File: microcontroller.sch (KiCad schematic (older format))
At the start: 52 parts, among them J3 FH12A-10S-0.5SH55, J4 , J5 Conn_ARM_JTAG_SWD_20, J6 26642801RP2, SW0 SW_Push, SW1 SW_Push, SW2 SW_Push, SW3 SW_Push, SW4 SW_Push, SW5 SW_Push, SW6 SW_Push, U7 EFM32GG942F1024

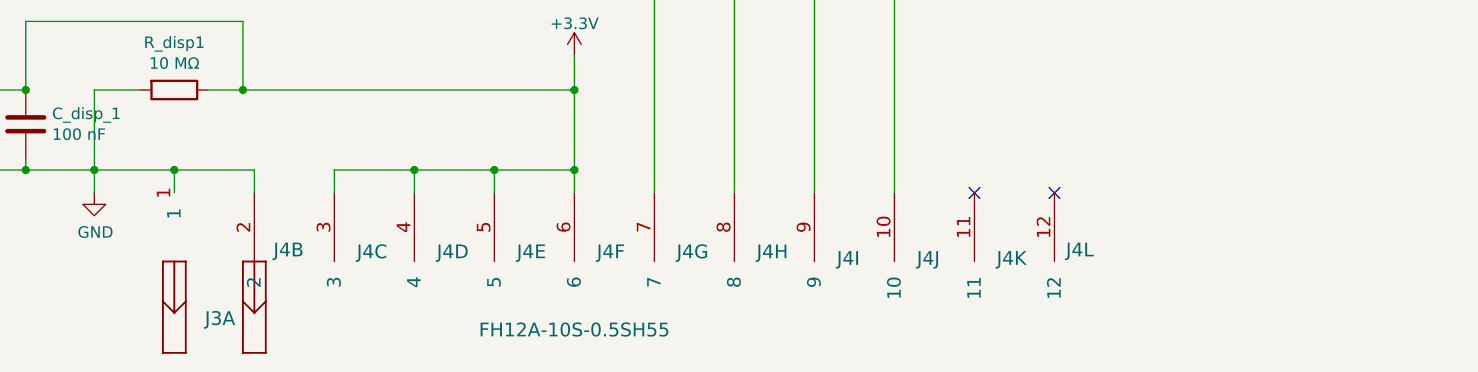
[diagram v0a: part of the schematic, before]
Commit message: Organize components and fix minor issues
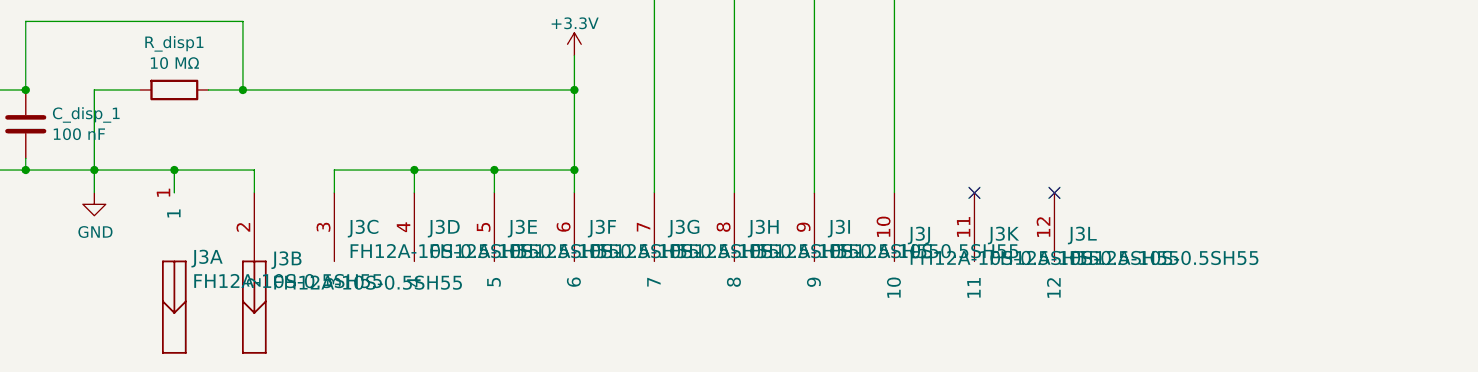
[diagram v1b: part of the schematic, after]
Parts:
- removed J4: (no value), Local:FH12A-10S-0.5SH55, symbol LCD:FH12A-10S-0.5SH55
- added unit 2 of J3
- added unit 3 of J3
- added unit 4 of J3
- added unit 5 of J3
- added unit 6 of J3
- added unit 7 of J3
- added unit 8 of J3
- added unit 9 of J3
- added unit 10 of J3
- added unit 11 of J3
- added unit 12 of J3
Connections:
- net +3V3: now also J3.3, J3.4, J3.5, J3.6
- net GND: now also J3.2
- net at U7.28 (PD0): now also J3.9
- net at U7.30 (PD2): now also J3.10
- net at U7.31 (PD3): now also J3.8
- net at J6.14: now also J3.7
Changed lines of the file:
@@
 	4400 6350 3800 6350
-$Comp
-L LCD:FH12A-10S-0.5SH55 J4
-U 2 1 5D873ACF
-P 4000 9050
-F 0 "J4" V 3750 9200 60  0000 C CNN
-F 1 " " V 4200 9050 60  0000 C CNN
-F 2 "Local:FH12A-10S-0.5SH55" H 4000 8990 60  0001 C CNN
-F 3 "" H 4000 9050 60  0000 C CNN
-	2    4000 9050
-	0    1    -1   0
-$EndComp
-$Comp
-L LCD:FH12A-10S-0.5SH55 J4
-U 3 1 5D88452F
-P 4350 9050
-F 0 "J4" V 4092 9148 60  0000 L CNN
-F 1 " " V 4198 9148 60  0000 L CNN
-F 2 "Local:FH12A-10S-0.5SH55" H 4350 8990 60  0001 C CNN
-F 3 "" H 4350 9050 60  0000 C CNN
-	3    4350 9050
-	0    1    -1   0
-$EndComp
-$Comp
-L LCD:FH12A-10S-0.5SH55 J4
-U 4 1 5D88BAB2
-P 4700 9050
-F 0 "J4" V 4442 9148 60  0000 L CNN
-F 1 " " V 4548 9148 60  0000 L CNN
-F 2 "Local:FH12A-10S-0.5SH55" H 4700 8990 60  0001 C CNN
-F 3 "" H 4700 9050 60  0000 C CNN
-	4    4700 9050
-	0    1    -1   0
-$EndComp
-$Comp
-L LCD:FH12A-10S-0.5SH55 J4
-U 5 1 5D891720
-P 5050 9050
-F 0 "J4" V 4792 9148 60  0000 L CNN
-F 1 " " V 4898 9148 60  0000 L CNN
-F 2 "Local:FH12A-10S-0.5SH55" H 5050 8990 60  0001 C CNN
-F 3 "" H 5050 9050 60  0000 C CNN
-	5    5050 9050
-	0    1    -1   0
-$EndComp
-$Comp
-L LCD:FH12A-10S-0.5SH55 J4
-U 6 1 5D89776E
-P 5400 9050
-F 0 "J4" V 5142 9148 60  0000 L CNN
-F 1 " " V 5248 9148 60  0000 L CNN
-F 2 "Local:FH12A-10S-0.5SH55" H 5400 8990 60  0001 C CNN
-F 3 "" H 5400 9050 60  0000 C CNN
-	6    5400 9050
-	0    1    -1   0
-$EndComp
-$Comp
-L LCD:FH12A-10S-0.5SH55 J4
-U 7 1 5D89D729
-P 5750 9050
-F 0 "J4" V 5492 9147 60  0000 L CNN
-F 1 " " V 5598 9147 60  0000 L CNN
-F 2 "Local:FH12A-10S-0.5SH55" H 5750 8990 60  0001 C CNN
-F 3 "" H 5750 9050 60  0000 C CNN
-	7    5750 9050
-	0    1    -1   0
-$EndComp
-$Comp
-L LCD:FH12A-10S-0.5SH55 J4
-U 8 1 5D8A2C47
-P 6100 9050
-F 0 "J4" V 5842 9147 60  0000 L CNN
-F 1 " " V 5948 9147 60  0000 L CNN
-F 2 "Local:FH12A-10S-0.5SH55" H 6100 8990 60  0001 C CNN
-F 3 "" H 6100 9050 60  0000 C CNN
-	8    6100 9050
-	0    1    -1   0
-$EndComp
-$Comp
-L LCD:FH12A-10S-0.5SH55 J4
-U 9 1 5D8AB529
-P 6450 9050
-F 0 "J4" V 6163 9148 60  0000 L CNN
-F 1 " " V 6269 9148 60  0000 L CNN
-F 2 "Local:FH12A-10S-0.5SH55" H 6450 8990 60  0001 C CNN
-F 3 "" H 6450 9050 60  0000 C CNN
-	9    6450 9050
-	0    1    -1   0
-$EndComp
-$Comp
-L LCD:FH12A-10S-0.5SH55 J4
-U 10 1 5D8B1A3C
-P 6800 9050
-F 0 "J4" V 6513 9148 60  0000 L CNN
-F 1 " " V 6619 9148 60  0000 L CNN
-F 2 "Local:FH12A-10S-0.5SH55" H 6800 8990 60  0001 C CNN
-F 3 "" H 6800 9050 60  0000 C CNN
-	10   6800 9050
-	0    1    -1   0
-$EndComp
-$Comp
-L LCD:FH12A-10S-0.5SH55 J4
-U 11 1 5D8B82A9
-P 7150 9050
-F 0 "J4" V 6863 9147 60  0000 L CNN
-F 1 " " V 6969 9147 60  0000 L CNN
-F 2 "Local:FH12A-10S-0.5SH55" H 7150 8990 60  0001 C CNN
-F 3 "" H 7150 9050 60  0000 C CNN
-	11   7150 9050
-	0    1    -1   0
-$EndComp
 $Comp
 L power:GND #PWR0139
@@
 	1    3300 9050
 	1    0    0    -1
-$EndComp
-$Comp
-L LCD:FH12A-10S-0.5SH55 J3
-U 1 1 5D85CD0B
-P 3650 9050
-F 0 "J3" V 3100 9250 60  0000 C CNN
-F 1 "FH12A-10S-0.5SH55" V 3050 10800 60  0000 C CNN
-F 2 "Local:FH12A-10S-0.5SH55" H 3650 8990 60  0001 C CNN
-F 3 "" H 3650 9050 60  0000 C CNN
-	1    3650 9050
-	0    1    -1   0
 $EndComp
 Wire Wire Line
@@
 	4000 9050 4000 8950
 $Comp
-L LCD:FH12A-10S-0.5SH55 J4
-U 12 1 5D9B45F3
-P 7500 9050
-F 0 "J4" V 7250 9000 60  0000 R CNN
-F 1 " " V 7213 8988 60  0000 R CNN
-F 2 "Local:FH12A-10S-0.5SH55" H 7500 8990 60  0001 C CNN
-F 3 "" H 7500 9050 60  0000 C CNN
-	12   7500 9050
-	0    -1   -1   0
-$EndComp
-$Comp
 L button:FSMSMTR SW0
 U 1 1 5DC135E8
@@
 Wire Wire Line
 	4150 6400 14400 6400
+$Comp
+L LCD:FH12A-10S-0.5SH55 J3
+U 1 1 5DA30D46
+P 3650 9050
+F 0 "J3" V 3368 8971 60  0000 R CNN
+F 1 "FH12A-10S-0.5SH55" V 3262 8971 60  0000 R CNN
+F 2 "Local:FH12A-10S-0.5SH55" H 3650 8990 60  0001 C CNN
+F 3 "" H 3650 9050 60  0000 C CNN
+	1    3650 9050
+	0    -1   -1   0
+$EndComp
+$Comp
+L LCD:FH12A-10S-0.5SH55 J3
+U 2 1 5DA525ED
+P 4000 9050
+F 0 "J3" V 3711 8971 60  0000 R CNN
+F 1 "FH12A-10S-0.5SH55" V 3605 8971 60  0000 R CNN
+F 2 "Local:FH12A-10S-0.5SH55" H 4000 8990 60  0001 C CNN
+F 3 "" H 4000 9050 60  0000 C CNN
+	2    4000 9050
+	0    -1   -1   0
+$EndComp
+$Comp
+L LCD:FH12A-10S-0.5SH55 J3
+U 3 1 5DA5397D
+P 4350 9050
+F 0 "J3" V 4199 8987 60  0000 R CNN
+F 1 "FH12A-10S-0.5SH55" V 4093 8987 60  0000 R CNN
+F 2 "Local:FH12A-10S-0.5SH55" H 4350 8990 60  0001 C CNN
+F 3 "" H 4350 9050 60  0000 C CNN
+	3    4350 9050
+	0    -1   -1   0
+$EndComp
+$Comp
+L LCD:FH12A-10S-0.5SH55 J3
+U 4 1 5DA7518D
+P 4700 9050
+F 0 "J3" V 4549 8987 60  0000 R CNN
+F 1 "FH12A-10S-0.5SH55" V 4443 8987 60  0000 R CNN
+F 2 "Local:FH12A-10S-0.5SH55" H 4700 8990 60  0001 C CNN
+F 3 "" H 4700 9050 60  0000 C CNN
+	4    4700 9050
+	0    -1   -1   0
+$EndComp
+$Comp
+L LCD:FH12A-10S-0.5SH55 J3
+U 5 1 5DA769A9
+P 5050 9050
+F 0 "J3" V 4899 8987 60  0000 R CNN
+F 1 "FH12A-10S-0.5SH55" V 4793 8987 60  0000 R CNN
+F 2 "Local:FH12A-10S-0.5SH55" H 5050 8990 60  0001 C CNN
+F 3 "" H 5050 9050 60  0000 C CNN
+	5    5050 9050
+	0    -1   -1   0
+$EndComp
+$Comp
+L LCD:FH12A-10S-0.5SH55 J3
+U 6 1 5DA7DC54
+P 5400 9050
+F 0 "J3" V 5249 8987 60  0000 R CNN
+F 1 "FH12A-10S-0.5SH55" V 5143 8987 60  0000 R CNN
+F 2 "Local:FH12A-10S-0.5SH55" H 5400 8990 60  0001 C CNN
+F 3 "" H 5400 9050 60  0000 C CNN
+	6    5400 9050
+	0    -1   -1   0
+$EndComp
+$Comp
+L LCD:FH12A-10S-0.5SH55 J3
+U 7 1 5DA7F197
+P 5750 9050
+F 0 "J3" V 5599 8987 60  0000 R CNN
+F 1 "FH12A-10S-0.5SH55" V 5493 8987 60  0000 R CNN
+F 2 "Local:FH12A-10S-0.5SH55" H 5750 8990 60  0001 C CNN
+F 3 "" H 5750 9050 60  0000 C CNN
+	7    5750 9050
+	0    -1   -1   0
+$EndComp
+$Comp
+L LCD:FH12A-10S-0.5SH55 J3
+U 8 1 5DA80692
+P 6100 9050
+F 0 "J3" V 5949 8987 60  0000 R CNN
+F 1 "FH12A-10S-0.5SH55" V 5843 8987 60  0000 R CNN
+F 2 "Local:FH12A-10S-0.5SH55" H 6100 8990 60  0001 C CNN
+F 3 "" H 6100 9050 60  0000 C CNN
+	8    6100 9050
+	0    -1   -1   0
+$EndComp
+$Comp
+L LCD:FH12A-10S-0.5SH55 J3
+U 9 1 5DA81DB1
+P 6450 9050
+F 0 "J3" V 6299 8987 60  0000 R CNN
+F 1 "FH12A-10S-0.5SH55" V 6193 8987 60  0000 R CNN
+F 2 "Local:FH12A-10S-0.5SH55" H 6450 8990 60  0001 C CNN
+F 3 "" H 6450 9050 60  0000 C CNN
+	9    6450 9050
+	0    -1   -1   0
+$EndComp
+$Comp
+L LCD:FH12A-10S-0.5SH55 J3
+U 10 1 5DA82F1D
+P 6800 9050
+F 0 "J3" V 6619 8987 60  0000 R CNN
+F 1 "FH12A-10S-0.5SH55" V 6513 8987 60  0000 R CNN
+F 2 "Local:FH12A-10S-0.5SH55" H 6800 8990 60  0001 C CNN
+F 3 "" H 6800 9050 60  0000 C CNN
+	10   6800 9050
+	0    -1   -1   0
+$EndComp
+$Comp
+L LCD:FH12A-10S-0.5SH55 J3
+U 11 1 5DA84636
+P 7150 9050
+F 0 "J3" V 6969 8987 60  0000 R CNN
+F 1 "FH12A-10S-0.5SH55" V 6863 8987 60  0000 R CNN
+F 2 "Local:FH12A-10S-0.5SH55" H 7150 8990 60  0001 C CNN
+F 3 "" H 7150 9050 60  0000 C CNN
+	11   7150 9050
+	0    -1   -1   0
+$EndComp
+$Comp
+L LCD:FH12A-10S-0.5SH55 J3
+U 12 1 5DA85E89
+P 7500 9050
+F 0 "J3" V 7319 8987 60  0000 R CNN
+F 1 "FH12A-10S-0.5SH55" V 7213 8987 60  0000 R CNN
+F 2 "Local:FH12A-10S-0.5SH55" H 7500 8990 60  0001 C CNN
+F 3 "" H 7500 9050 60  0000 C CNN
+	12   7500 9050
+	0    -1   -1   0
+$EndComp
 $EndSCHEMATC
